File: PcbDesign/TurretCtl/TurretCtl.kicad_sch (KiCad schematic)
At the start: 7 parts, among them J1 PWR, J2 St1, J3 St2, J4 Sv1, J5 Sense, J6 Sv2

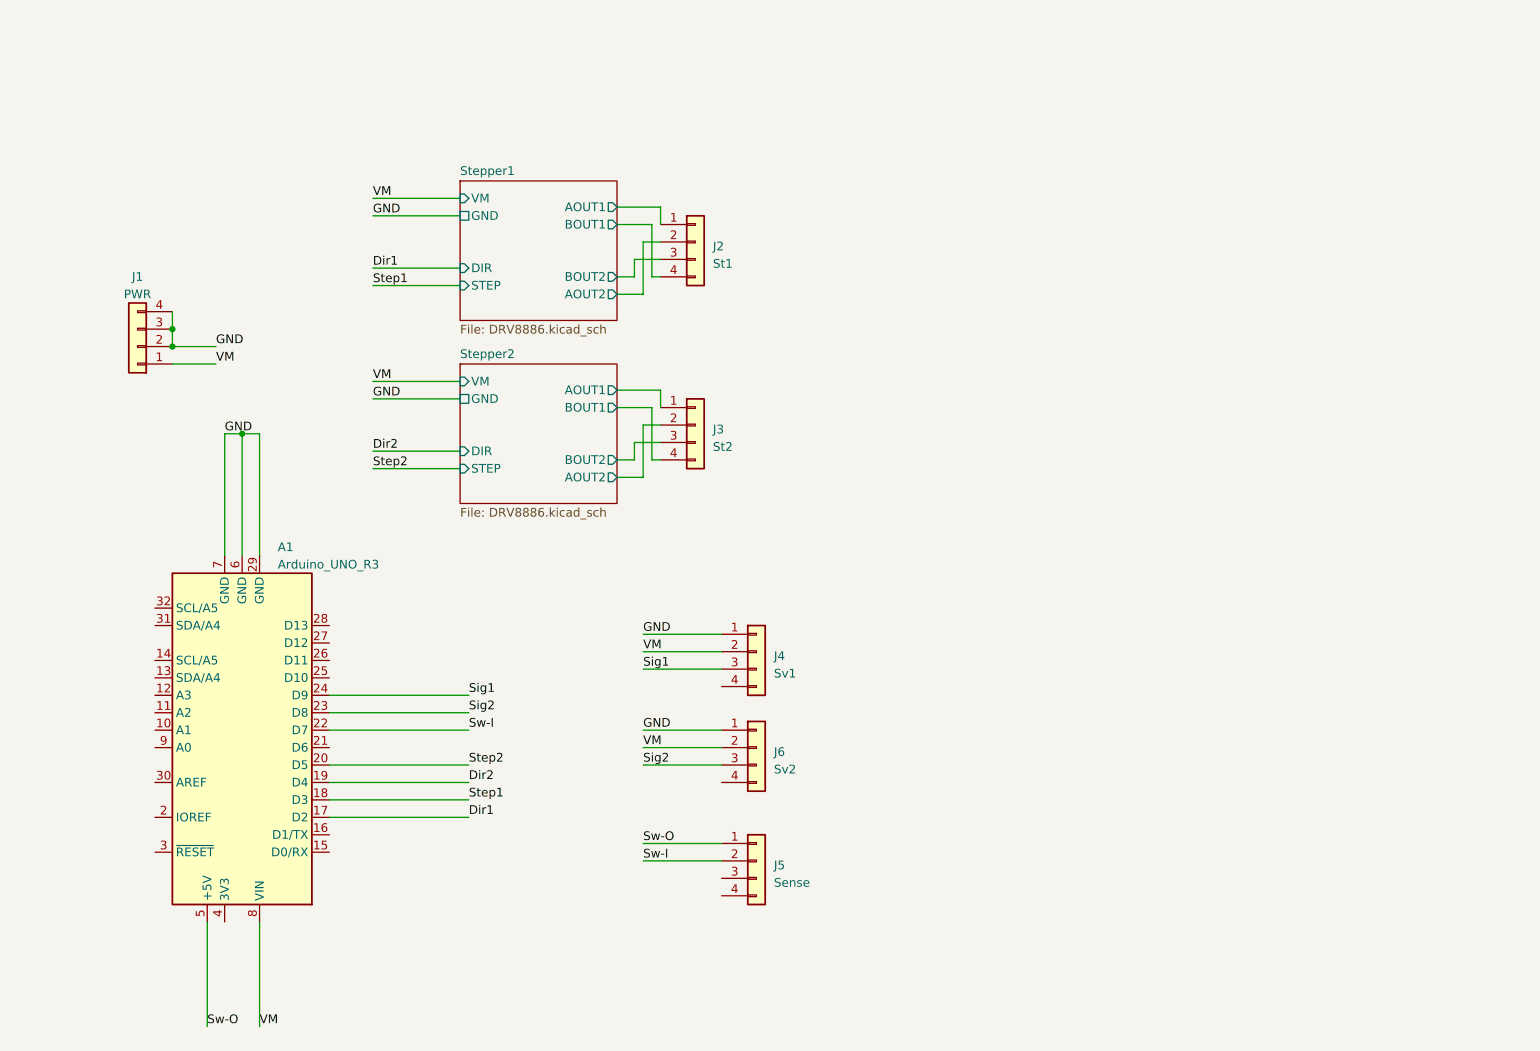
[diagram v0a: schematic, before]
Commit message: TurretCtl V2
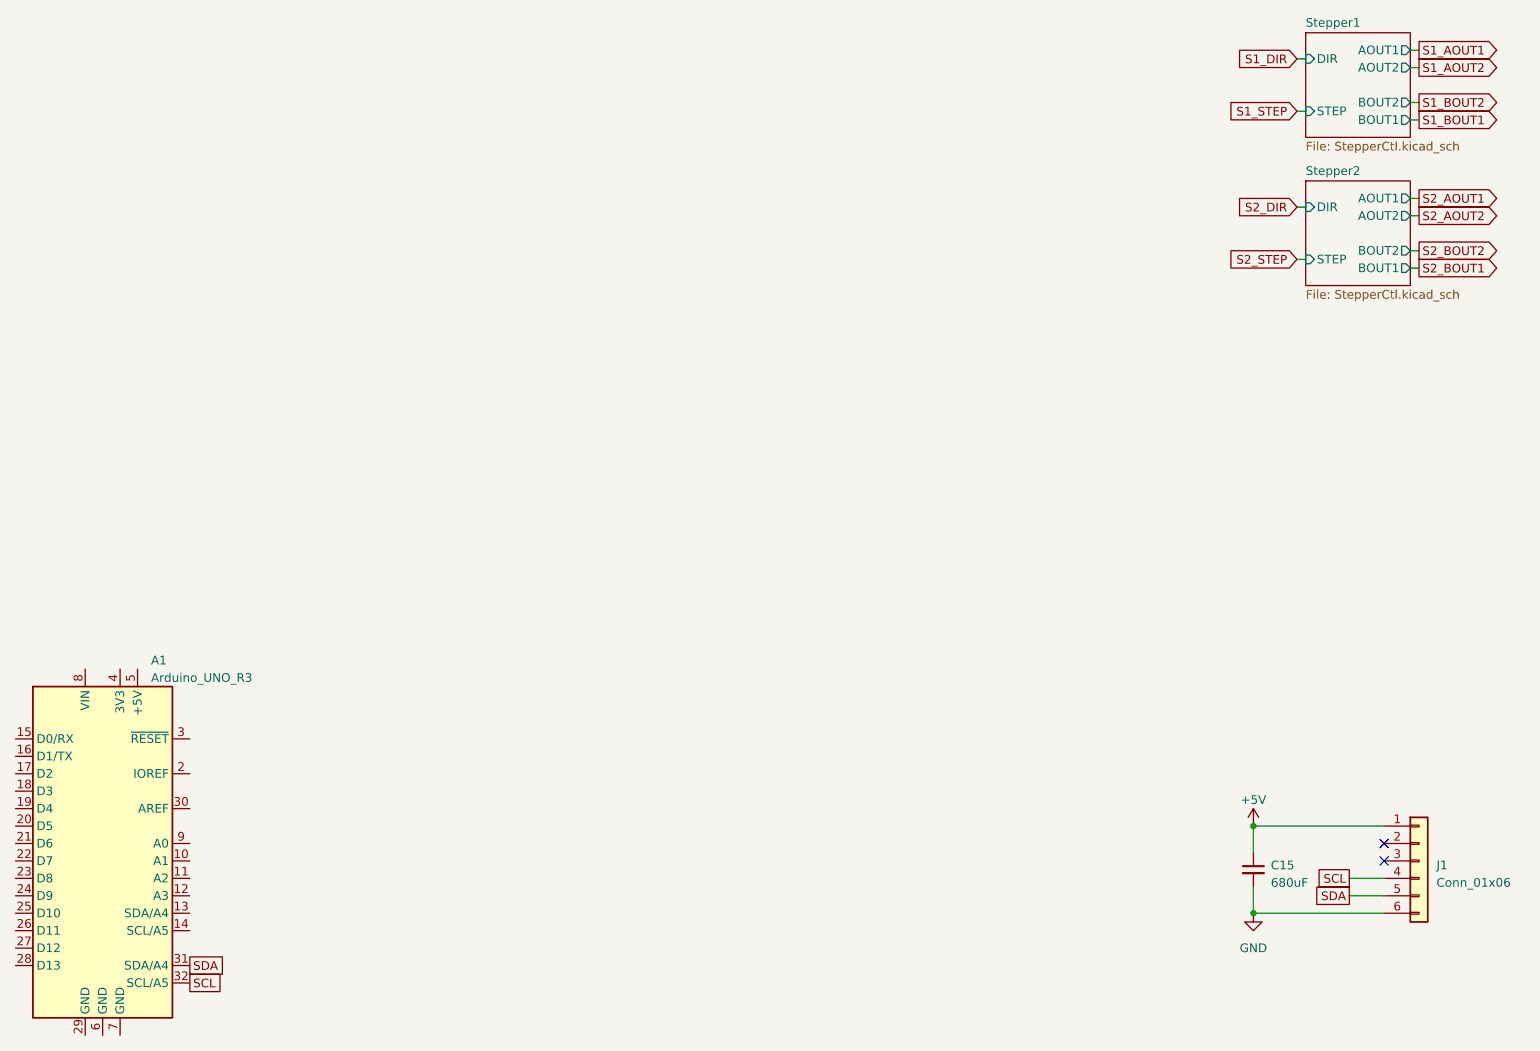
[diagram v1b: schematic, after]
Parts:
- removed J1: PWR, TerminalBlock_Phoenix:TerminalBlock_Phoenix_PTSM-0,5-4-2.5-H-THR_1x04_P2.50mm_Horizontal, symbol Connector_Generic:Conn_01x04
- removed J2: St1, TerminalBlock_Phoenix:TerminalBlock_Phoenix_PTSM-0,5-4-2.5-H-THR_1x04_P2.50mm_Horizontal, symbol Connector_Generic:Conn_01x04
- removed J3: St2, TerminalBlock_Phoenix:TerminalBlock_Phoenix_PTSM-0,5-4-2.5-H-THR_1x04_P2.50mm_Horizontal, symbol Connector_Generic:Conn_01x04
- removed J4: Sv1, TerminalBlock_Phoenix:TerminalBlock_Phoenix_PTSM-0,5-4-2.5-H-THR_1x04_P2.50mm_Horizontal, symbol Connector_Generic:Conn_01x04
- removed J5: Sense, TerminalBlock_Phoenix:TerminalBlock_Phoenix_PTSM-0,5-4-2.5-H-THR_1x04_P2.50mm_Horizontal, symbol Connector_Generic:Conn_01x04
- removed J6: Sv2, TerminalBlock_Phoenix:TerminalBlock_Phoenix_PTSM-0,5-4-2.5-H-THR_1x04_P2.50mm_Horizontal, symbol Connector_Generic:Conn_01x04
- added C15: 680uF, symbol Device:C_Small
- added J1: Conn_01x06, symbol Connector_Generic:Conn_01x06
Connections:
- net GND: now also C15.2, J1.6 (Pin_6); no longer A1.29 (GND), A1.6 (GND), A1.7 (GND)
- net SDA: now reaches A1.31 (SDA/A4)
- net SDA: now also J1.5 (Pin_5)
- net SCL: now reaches A1.32 (SCL/A5)
- net SCL: now also J1.4 (Pin_4)
- net Dir1: no longer names the net of A1.17 (D2)
- net Dir2: no longer names the net of A1.19 (D4)
- net Sig1: no longer names the net of A1.24 (D9)
- net Sig2: no longer names the net of A1.23 (D8)
- net Step1: no longer names the net of A1.18 (D3)
- net Step2: no longer names the net of A1.20 (D5)
- net Sw-I: no longer names the net of A1.22 (D7)
- net Sw-O: no longer names the net of A1.5 (+5V)
- net VM: no longer names the net of A1.8 (VIN)
- new net +5V: C15.1, J1.1 (Pin_1)
- no-connect marks 0 -> 2
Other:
- sheet Stepper1: file DRV8886.kicad_sch -> StepperCtl.kicad_sch
- sheet Stepper1 ports: added none; removed GND, VM
- sheet Stepper2: file DRV8886.kicad_sch -> StepperCtl.kicad_sch
- sheet Stepper2 ports: added none; removed GND, VM
